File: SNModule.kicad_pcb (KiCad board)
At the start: 2 copper layers, 78.2 x 125 mm, 68 parts, among them J1 DB9_Male_MountingHoles, J10 TBL009-254-02GY-2GY, J11 Conn_01x04, J12 Conn_01x04, J13 Conn_01x04, J14 Conn_01x02, J2 DB9_Female_MountingHoles, J3 TBL009-254-02GY-2GY, J4 TBL009-254-02GY-2GY, J5 TBL009-254-02GY-2GY, J6 TBL009-254-02GY-2GY, J7 TBL009-254-02GY-2GY, J8 TBL009-254-02GY-2GY, J9 TBL009-254-02GY-2GY, Q1 KSC1815, SW2 SW_Push, SW3 SW_Push, U1 Teensy4.0, U2 MCP2562-E-P, U3 MCP2562-E-P, U4 FM24C64B, U5 MCP3008, U6 TSR_1-2450, U7 EN11-HSM1AF15

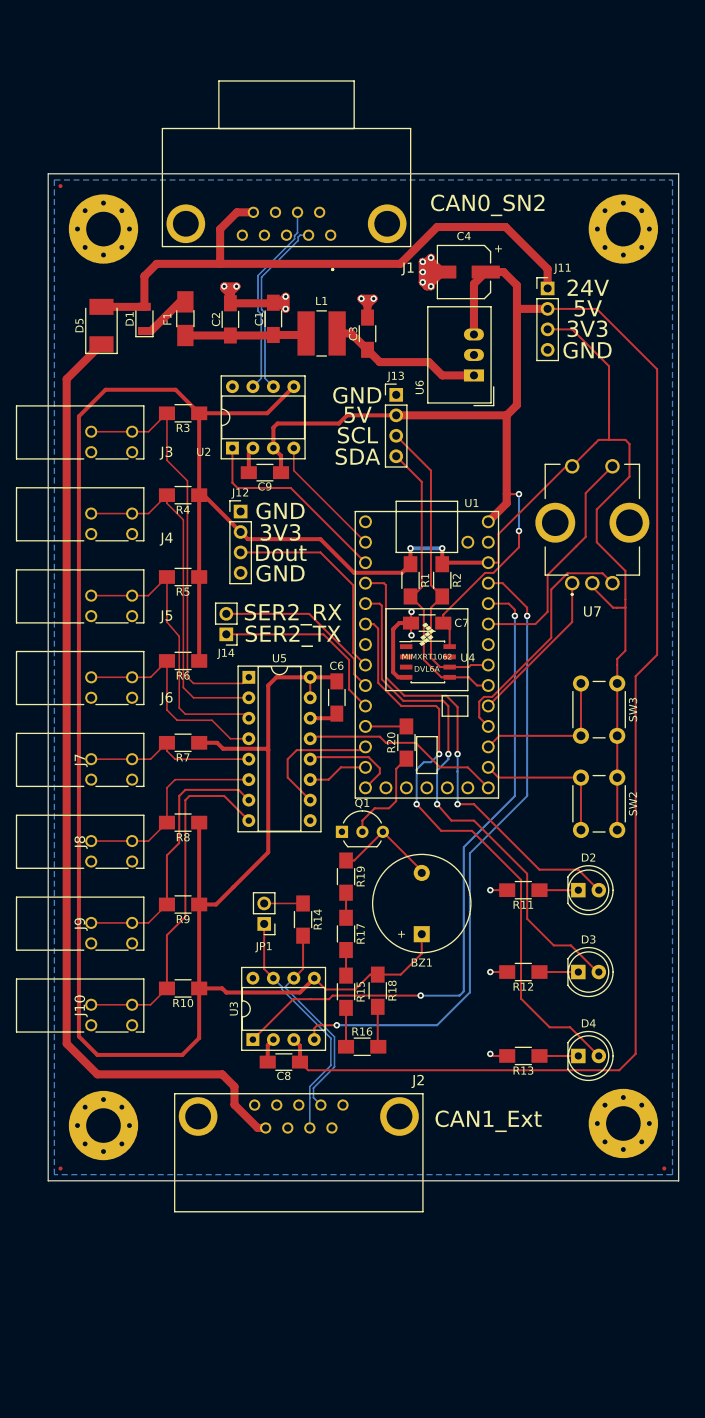
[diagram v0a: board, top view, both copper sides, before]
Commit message: Rev1
Orderd and ariving soon
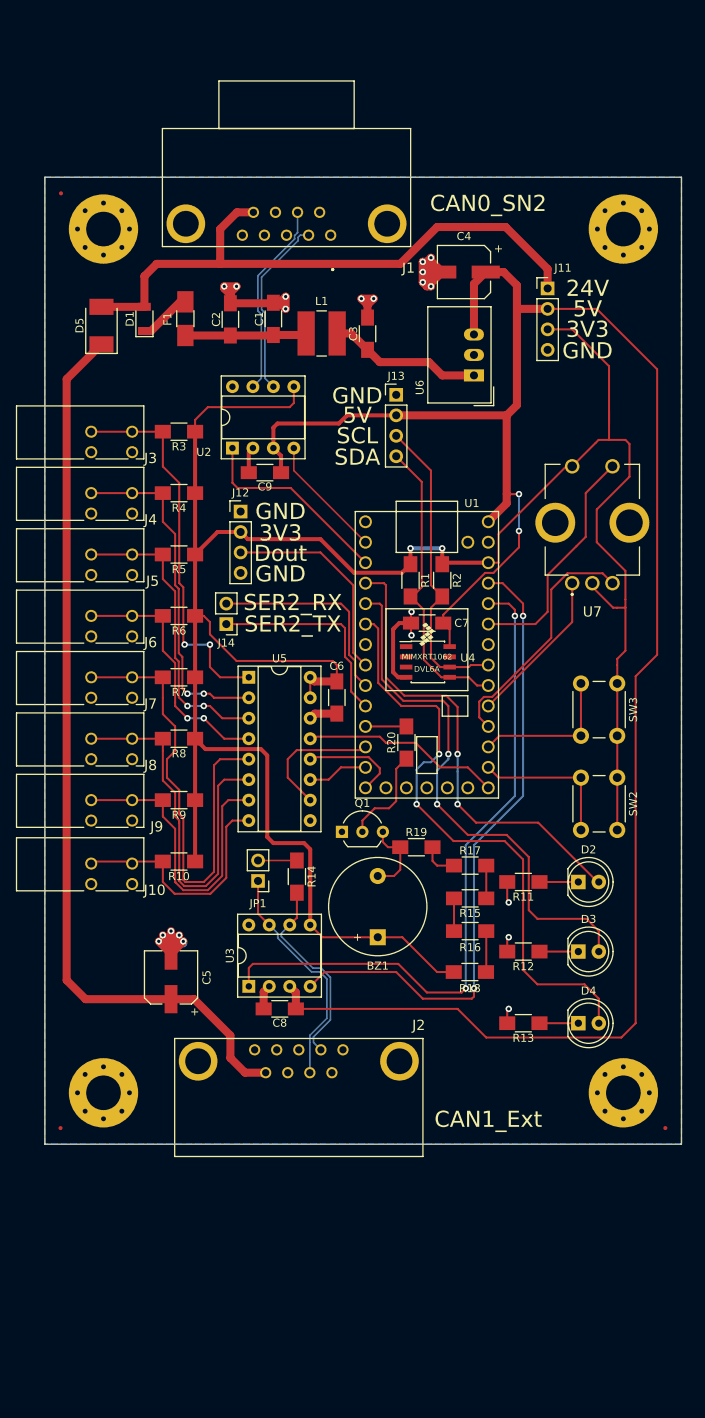
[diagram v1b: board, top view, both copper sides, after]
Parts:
- added C5: 100uF, Capacitors_SMD:CP_Elec_6.3x7.7, F.Cu at (41.7, 136.3)
- moved R16 19.6 mm to (78.8, 130.6)
- moved R15 19.3 mm to (78.8, 126.5), turned to 180 degrees
- moved R17 17.6 mm to (78.8, 122.4), turned to 0 degrees
- moved J10 17.5 mm to (31.8, 122.2)
- moved R10 15.8 mm to (42.6, 121.9)
- moved J9 15.2 mm to (31.8, 114.3)
- moved R9 13.0 mm to (42.6, 114.3)
- moved J8 12.7 mm to (31.8, 106.7)
- moved R18 11.7 mm to (78.7, 135.6), turned to 0 degrees
- moved R8 10.4 mm to (42.6, 106.7)
- moved J7 10.2 mm to (31.8, 99.1)
- moved R19 9.46 mm to (72.1, 120.1), turned to 0 degrees
- moved R7 8.14 mm to (42.6, 99.1)
- moved J6 7.62 mm to (31.8, 91.4)
- moved J2 6.86 mm to (63.0, 145.3)
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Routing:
- net +3V3: track 427.3 -> 302.8 mm
- net Net-(J7-Pad1): track 21.8 -> 58.2 mm
- net Net-(J8-Pad1): track 25.2 -> 48.2 mm
- net Net-(J10-Pad1): track 43.9 -> 30.2 mm
- net GND: track 68.0 -> 80.7 mm, vias 16 -> 21
- net Net-(C5-Pad1): track 119.3 -> 112.1 mm
- net Net-(J9-Pad1): track 33.9 -> 38.9 mm
- net Net-(J3-Pad1): track 52.4 -> 47.7 mm, vias 0 -> 2
- net SERIAL2_RX: track 22.1 -> 25.6 mm
- net Net-(J6-Pad1): track 28.0 -> 31.5 mm, vias 0 -> 2
- net Net-(BZ1-Pad2): track 13.1 -> 9.60 mm
- net SERIAL2_TX: track 23.1 -> 25.6 mm
- net +5V: track 257.2 -> 254.8 mm
- net Mod_CAN1_TX: track 82.3 -> 84.2 mm
- net Net-(R17-Pad1): track 3.11 -> 4.62 mm
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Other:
- board size 78.2 x 125 mm -> 79 x 120 mm
- net class Power added: clearance 0.2, trace_width 0.25, via_dia 0.8, via_drill 0.5
- rule pad_to_mask_clearance: 0.051 -> 0.05
- rule solder_mask_min_width: 0.25 -> 0.2
- rule via_min_size: 0.4 -> 0.5
- board text added: "JLCJLCJLCJLC"
- board text added: "SN2 Extension Rev 1"

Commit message: Rev2 done
Orderd and Assembeld PCB, works sofar, no magic Smoke sofar :D
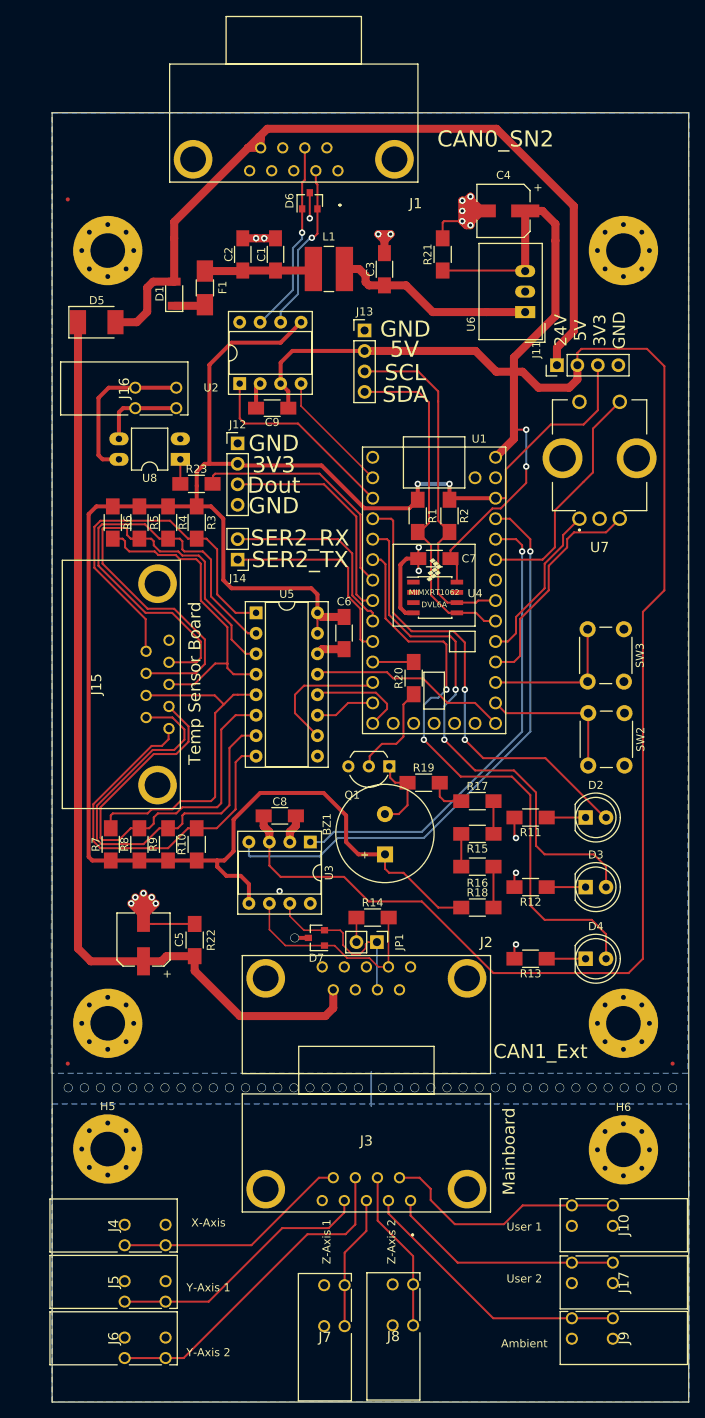
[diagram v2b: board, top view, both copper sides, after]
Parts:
- added D6: CDSOT23-T24CAN, TO_SOT_Packages_SMD:SOT-23, F.Cu at (58.9, 39.9)
- added D7: CDSOT23-T24CAN, TO_SOT_Packages_SMD:SOT-23, F.Cu at (59.7, 131.4)
- added H5: MountingHole_Pad, Mounting_Holes:MountingHole_4.3mm_M4_Pad_Via, F.Cu at (33.8, 157.6)
- added H6: MountingHole_Pad, Mounting_Holes:MountingHole_4.3mm_M4_Pad_Via, F.Cu at (97.8, 157.7)
- added J15: DB9_Female_MountingHoles, SamacSys_Parts:D09S23A4GV00LF, F.Cu at (41.4, 105.4)
- added J16: TBL009-254-02GY-2GY, SamacSys_Parts:TBL00925402GY2GY, F.Cu at (37.2, 63.1)
- added J17: TBL009-254-02GY-2GY, SamacSys_Parts:TBL00925402GY2GY, F.Cu at (96.5, 174.2)
- added R21: 1M, Resistors_SMD:R_1206_HandSoldering, F.Cu at (75.4, 46.6)
- added R22: 1M, Resistors_SMD:R_1206_HandSoldering, F.Cu at (44.6, 131.7)
- added R23: 120R, Resistors_SMD:R_1206_HandSoldering, F.Cu at (44.8, 75.1)
- added U8: TLP785, Housings_DIP:DIP-4_W7.62mm_LongPads, F.Cu at (42.8, 72.0)
- BZ1: footprint Buzzers_Beepers:Buzzer_12x9.5RM7.6 -> Blanket Github additions:Buzzer_TDK_12.2x6.5RM5
- J3: value TBL009-254-02GY-2GY -> DB9_Male_MountingHoles; footprint SamacSys_Parts:TBL00925402GY2GY -> SamacSys_Parts:D09P23A4GV00LF
- Q1: value KSC1815 -> BC337
- R10, R9: value Res -> 27k
- moved J3 103.3 mm to (71.4, 164.0), turned to 180 degrees
- moved J9 93.0 mm to (96.5, 181.1), turned to 90 degrees
- moved J4 90.9 mm to (35.9, 167.0)
- moved J5 90.3 mm to (35.9, 174.0)
- moved J6 89.7 mm to (35.9, 181.0)
- moved J7 85.6 mm to (60.7, 179.6), turned to 0 degrees
- moved J8 81.8 mm to (69.2, 179.5), turned to 0 degrees
- moved J10 78.8 mm to (96.5, 167.1), turned to 90 degrees
- moved C8 24.0 mm to (55.1, 116.2), turned to 0 degrees
- moved R7 22.4 mm to (34.2, 119.8), turned to 90 degrees
- moved U3 19.5 mm to (58.9, 119.5), turned to 270 degrees
- moved JP1 16.6 mm to (67.2, 131.9), turned to 270 degrees
- moved R6 14.2 mm to (34.4, 79.9), turned to 270 degrees
- moved R8 14.0 mm to (37.7, 119.8), turned to 90 degrees
- moved J2 13.3 mm to (71.4, 135.0)
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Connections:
- J10 pad 1: Net-(J10-Pad1) -> GND
- J10 pad 2: Net-(J10-Pad1) -> GND
- J10 pad 3: GND -> Net-(J10-Pad3)
- J10 pad 4: GND -> Net-(J10-Pad3)
- J3 pad 1: Net-(J3-Pad1) -> Net-(J17-Pad3)
- J3 pad 2: Net-(J3-Pad1) -> Net-(J3-Pad2)
- J3 pad 3: GND -> Net-(J3-Pad3)
- J3 pad 4: GND -> Net-(J3-Pad4)
- J4 pad 1: Net-(J4-Pad1) -> GND
- J4 pad 2: Net-(J4-Pad1) -> GND
- J4 pad 3: GND -> Net-(J3-Pad9)
- J4 pad 4: GND -> Net-(J3-Pad9)
- J5 pad 1: Net-(J5-Pad1) -> GND
- J5 pad 2: Net-(J5-Pad1) -> GND
- J5 pad 3: GND -> Net-(J3-Pad4)
- J5 pad 4: GND -> Net-(J3-Pad4)
- J6 pad 1: Net-(J6-Pad1) -> GND
- J6 pad 2: Net-(J6-Pad1) -> GND
- J6 pad 3: GND -> Net-(J3-Pad8)
- J6 pad 4: GND -> Net-(J3-Pad8)
- J7 pad 1: Net-(J7-Pad1) -> GND
- J7 pad 2: Net-(J7-Pad1) -> GND
- J7 pad 3: GND -> Net-(J3-Pad3)
- J7 pad 4: GND -> Net-(J3-Pad3)
- J8 pad 1: Net-(J8-Pad1) -> GND
- J8 pad 2: Net-(J8-Pad1) -> GND
- J8 pad 3: GND -> Net-(J3-Pad7)
- J8 pad 4: GND -> Net-(J3-Pad7)
- J9 pad 1: Net-(J9-Pad1) -> GND
- J9 pad 2: Net-(J9-Pad1) -> GND
- J9 pad 3: GND -> Net-(J3-Pad2)
- J9 pad 4: GND -> Net-(J3-Pad2)
- Q1 pad 1: GND -> Net-(BZ1-Pad2)
- Q1 pad 3: Net-(BZ1-Pad2) -> GND
- R10 pad 2: Net-(J10-Pad1) -> Net-(J15-Pad1)
- R3 pad 2: Net-(J3-Pad1) -> Net-(J15-Pad9)
- R4 pad 2: Net-(J4-Pad1) -> Net-(J15-Pad4)
- R5 pad 2: Net-(J5-Pad1) -> Net-(J15-Pad8)
- R6 pad 2: Net-(J6-Pad1) -> Net-(J15-Pad3)
- R7 pad 2: Net-(J7-Pad1) -> Net-(J15-Pad7)
- R8 pad 2: Net-(J8-Pad1) -> Net-(J15-Pad2)
- R9 pad 2: Net-(J9-Pad1) -> Net-(J15-Pad6)
- SW2 pad 1: +3V3 -> GND
- SW3 pad 1: +3V3 -> GND
- U1 pad 7: Net-(U1-Pad7) -> Opto1
- U5 pad 1: Net-(J3-Pad1) -> Net-(J15-Pad9)
- U5 pad 2: Net-(J4-Pad1) -> Net-(J15-Pad4)
- U5 pad 3: Net-(J5-Pad1) -> Net-(J15-Pad8)
- U5 pad 4: Net-(J6-Pad1) -> Net-(J15-Pad3)
- U5 pad 5: Net-(J7-Pad1) -> Net-(J15-Pad7)
- U5 pad 6: Net-(J8-Pad1) -> Net-(J15-Pad2)
- U5 pad 7: Net-(J9-Pad1) -> Net-(J15-Pad6)
- U5 pad 8: Net-(J10-Pad1) -> Net-(J15-Pad1)
- U7 pad C1: +3V3 -> GND
- U7 pad D1: +3V3 -> GND
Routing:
- net Net-(J15-Pad8): track 0.00 -> 62.6 mm
- net Net-(J7-Pad1): track 58.2 -> 0.00 mm
- net Net-(J15-Pad4): track 0.00 -> 56.2 mm
- net Net-(J15-Pad6): track 0.00 -> 55.5 mm
- net Net-(J15-Pad2): track 0.00 -> 55.1 mm
- net Net-(J8-Pad1): track 48.2 -> 0.00 mm
- net Net-(J3-Pad1): track 47.7 -> 0.00 mm, vias 2 -> 0
- net Net-(J15-Pad1): track 0.00 -> 47.3 mm
- net Net-(J15-Pad9): track 0.00 -> 46.5 mm
- net +3V3: track 302.8 -> 257.2 mm
- net Net-(J4-Pad1): track 42.9 -> 0.00 mm, vias 2 -> 0
- net Net-(J15-Pad7): track 0.00 -> 42.1 mm
- net Net-(J3-Pad8): track 0.00 -> 41.3 mm
- net Net-(J15-Pad3): track 0.00 -> 39.2 mm
- net Net-(J9-Pad1): track 38.9 -> 0.00 mm
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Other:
- board size 79 x 120 mm -> 79 x 160 mm
- board text added: "24V 5V 3V3 GND"
- board text added: "Mainboard"
- board text added: "SN2 Extension Rev 2"
- board text added: "Temp Sensor Board"
- board text added: "User 1 User 2 Ambient"
- board text added: "X-Axis Y-Axis 1 Y-Axis 2"
- board text added: "Z-Axis 1 Z-Axis 2"
- board text removed: "24V"
- board text removed: "SN2 Extension Rev 1"
